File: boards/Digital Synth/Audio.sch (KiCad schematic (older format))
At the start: 33 parts, among them J1 AudioJack3, J2 AudioJack3, J3 DIN-5, J4 DIN-5, U2 6N138, U3 PCM5101A, U4 SN74LVC2G14

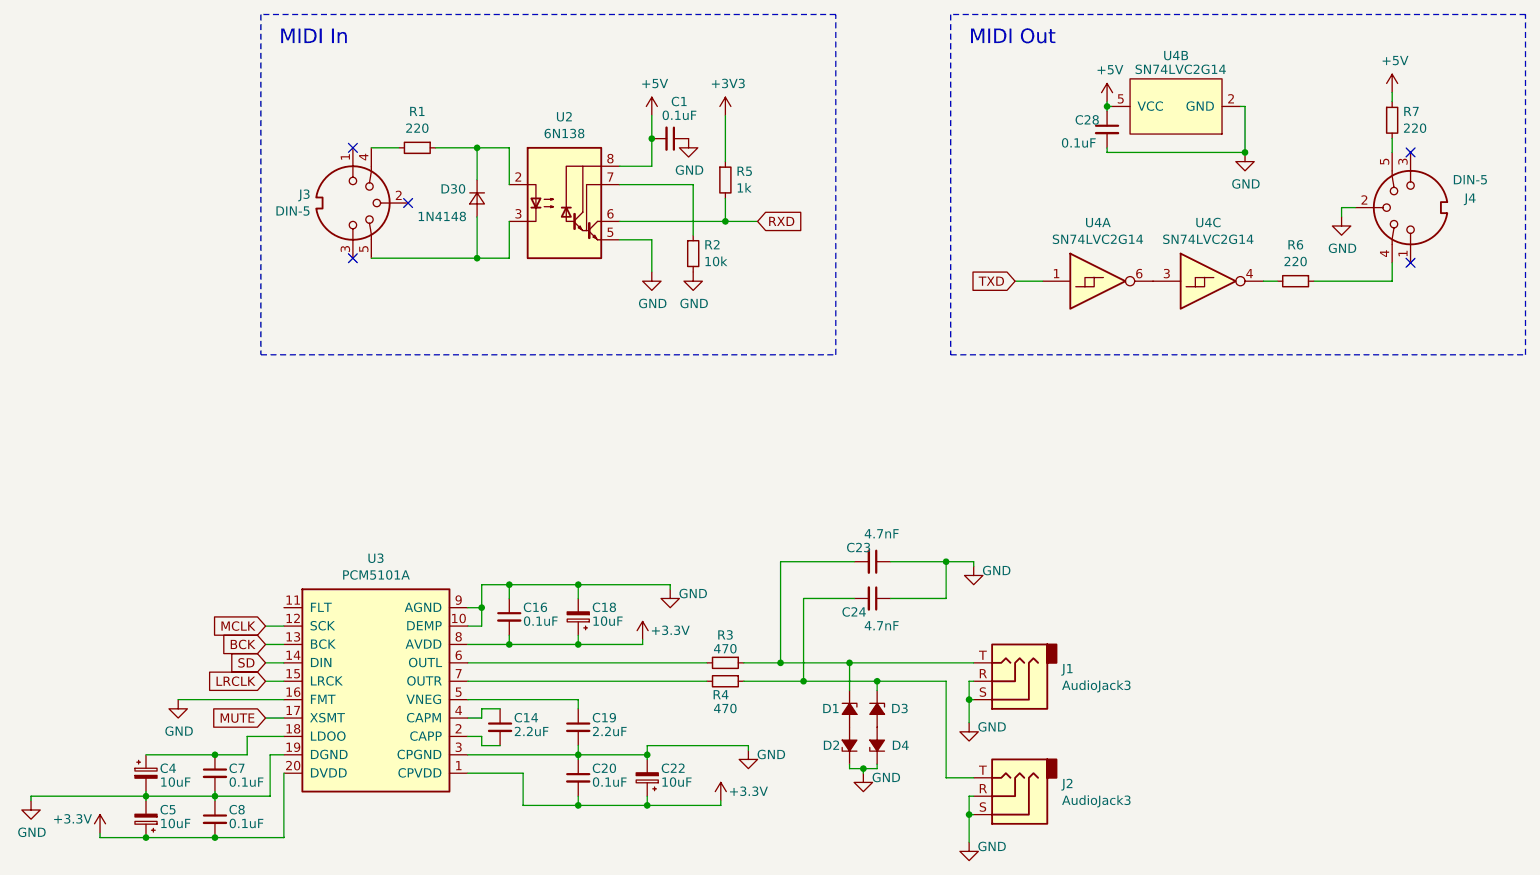
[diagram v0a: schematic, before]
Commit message: almost done with layout
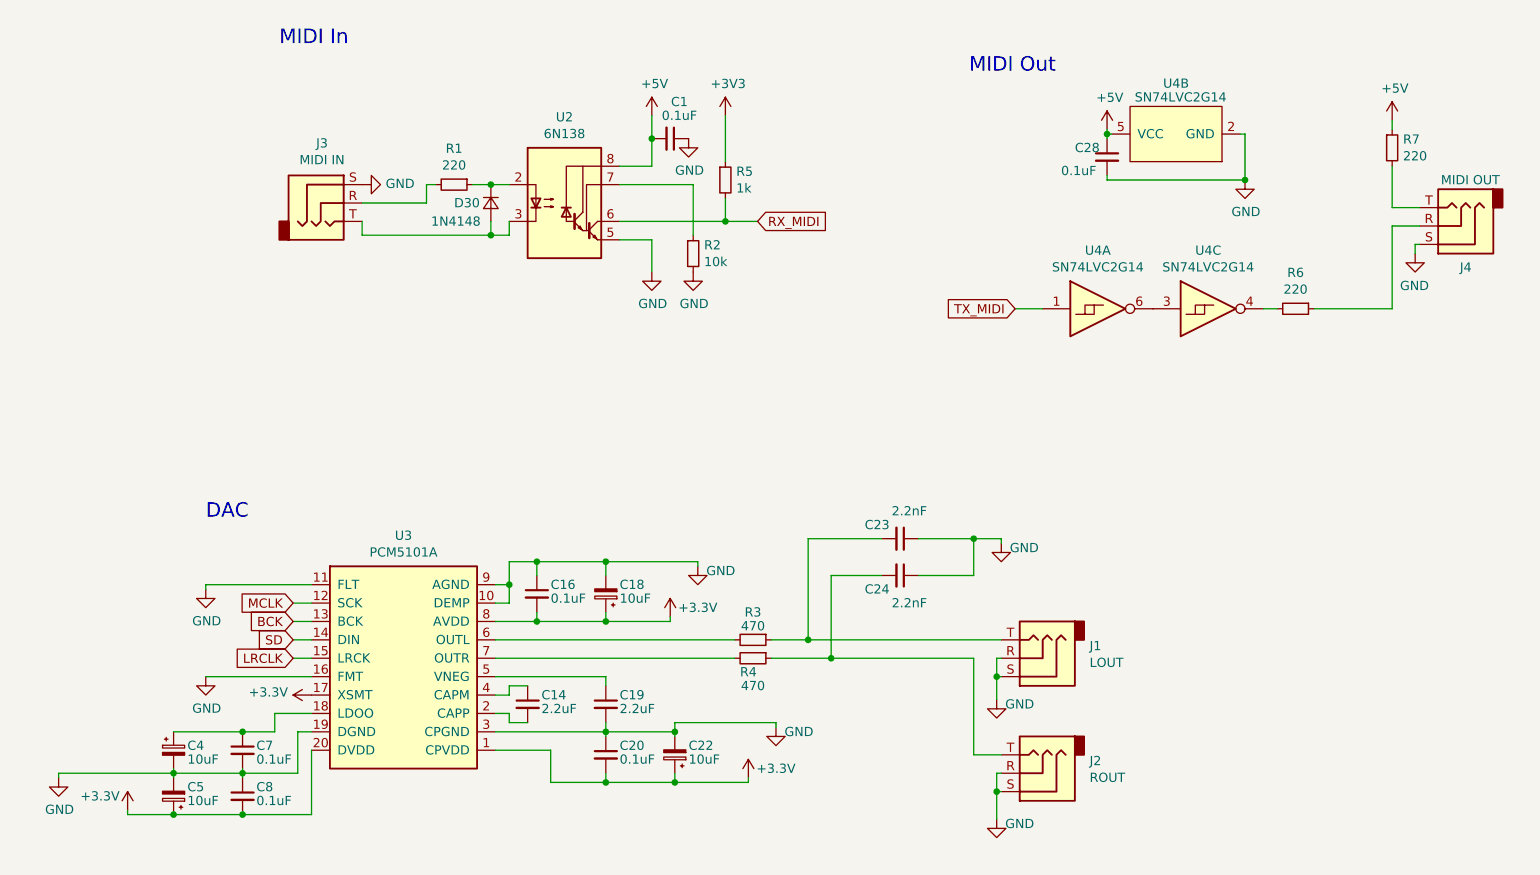
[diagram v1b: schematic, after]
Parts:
- removed D1, D2, D3, D4: D_Zener_Small_ALT, Diode_SMD:D_0805_2012Metric_Pad1.15x1.40mm_HandSolder, symbol device:D_Zener_Small_ALT
- removed J3, J4: DIN-5, Connector_Audio_Ext:MIDI_DIN5, symbol Connector:DIN-5_180degree
- added J3: MIDI IN, Connector_Audio:Jack_3.5mm_CUI_SJ1-3533NG_Horizontal, symbol Connector:AudioJack3
- added J4: MIDI OUT, Connector_Audio:Jack_3.5mm_CUI_SJ1-3533NG_Horizontal, symbol Connector:AudioJack3
- C23, C24: value 4.7nF -> 2.2nF; footprint Capacitor_SMD:C_0603_1608Metric_Pad1.05x0.95mm_HandSolder -> Capacitor_SMD:C_1206_3216Metric
- D30: footprint Diode_SMD:D_0805_2012Metric_Pad1.15x1.40mm_HandSolder -> Diode_SMD:D_SOD-323
- J1: value AudioJack3 -> LOUT; footprint Connector_Audio_Ext:Jack_6.35mm_Neutrik_NMJ4HFD2_Horizontal -> Connector_Audio:Jack_3.5mm_CUI_SJ1-3533NG_Horizontal
- J2: value AudioJack3 -> ROUT; footprint Connector_Audio_Ext:Jack_6.35mm_Neutrik_NMJ4HFD2_Horizontal -> Connector_Audio:Jack_3.5mm_CUI_SJ1-3533NG_Horizontal
- R1, R2, R5, R6, R7: footprint Resistor_SMD:R_0805_2012Metric_Pad1.15x1.40mm_HandSolder -> Resistor_SMD:R_0603_1608Metric_Pad1.05x0.95mm_HandSolder
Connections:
- net MUTE is gone; now on net +3V3: U3.17 (XSMT)
- net GND: now also U3.11 (FLT), J3.S, J4.S
- net at R6.1: now also J4.R
- net at R7.2: now also J4.T
- net at D30.2 (A), U2.3 (C2): now also J3.T
- net at R1.2: now also J3.R
- net RXD renamed RX_MIDI
- net TXD renamed TX_MIDI
- no-connect marks 5 -> 0
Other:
- note added: "DAC"
- moved on the sheet: C14, C16, C18, C19, C20, C22, C23, C24, C28, C4, C5, C7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

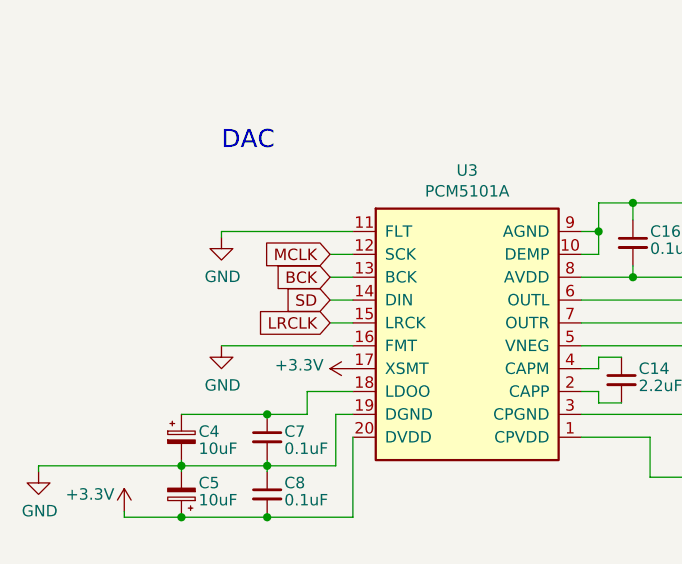
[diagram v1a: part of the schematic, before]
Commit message: finished layout
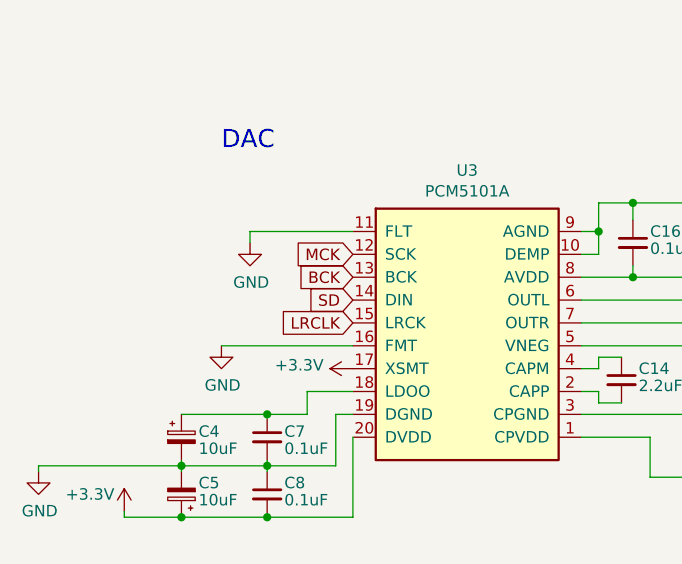
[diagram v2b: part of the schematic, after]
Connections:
- net MCLK renamed MCK
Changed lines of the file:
@@
 Comment4 ""
 $EndDescr
-Text GLabel 2700 4750 0    50   Input ~ 0
+Text GLabel 2800 4750 0    50   Input ~ 0
 SD
-Text GLabel 2700 4850 0    50   Input ~ 0
+Text GLabel 2800 4850 0    50   Input ~ 0
 LRCLK
-Text GLabel 2700 4650 0    50   Input ~ 0
+Text GLabel 2800 4650 0    50   Input ~ 0
 BCK
-Text GLabel 2700 4550 0    50   Input ~ 0
-MCLK
 Wire Wire Line
 	6525 5575 6525 5725
@@
 	1    0    0    -1
 $EndComp
-Wire Wire Line
-	2700 4850 2800 4850
-Wire Wire Line
-	2700 4750 2800 4750
-Wire Wire Line
-	2700 4650 2800 4650
-Wire Wire Line
-	2700 4550 2800 4550
 $Comp
 L Synth_Lib:PCM5101A U?
@@
 $EndComp
 Wire Wire Line
-	2800 4450 2225 4450
+	2800 4450 2350 4450
 $Comp
 L power:GND #PWR?
 U 1 1 6256264A
-P 2225 4475
+P 2350 4500
 AR Path="/6256264A" Ref="#PWR?"  Part="1"
 AR Path="/61FCD2FD/6256264A" Ref="#PWR0116"  Part="1"
-F 0 "#PWR0116" H 2225 4225 50  0001 C CNN
-F 1 "GND" H 2230 4302 50  0000 C CNN
-F 2 "" H 2225 4475 50  0001 C CNN
-F 3 "" H 2225 4475 50  0001 C CNN
-	1    2225 4475
-	1    0    0    -1
-$EndComp
-Wire Wire Line
-	2225 4450 2225 4475
+F 0 "#PWR0116" H 2350 4250 50  0001 C CNN
+F 1 "GND" H 2355 4327 50  0000 C CNN
+F 2 "" H 2350 4500 50  0001 C CNN
+F 3 "" H 2350 4500 50  0001 C CNN
+	1    2350 4500
+	1    0    0    -1
+$EndComp
+Wire Wire Line
+	2350 4450 2350 4500
+Text GLabel 2800 4550 0    50   Input ~ 0
+MCK
 $EndSCHEMATC
